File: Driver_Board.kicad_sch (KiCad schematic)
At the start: 26 parts, among them J1 200, J2 100, J3 10, J4 Conn_01x04, J5 Conn_01x04, J6 Control

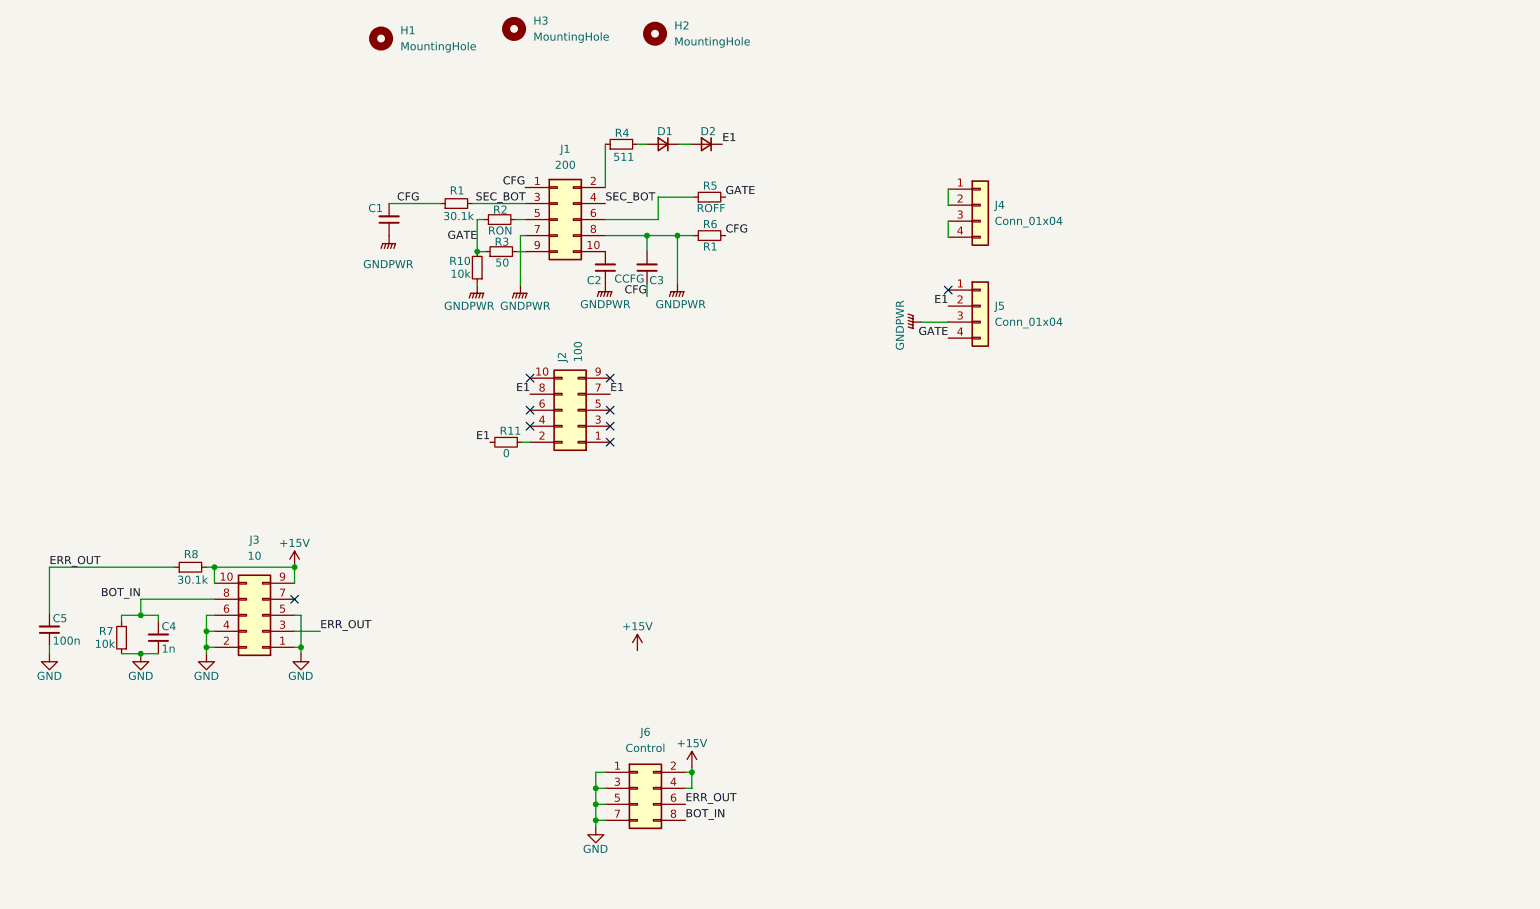
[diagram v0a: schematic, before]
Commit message: Основа ADUM4135
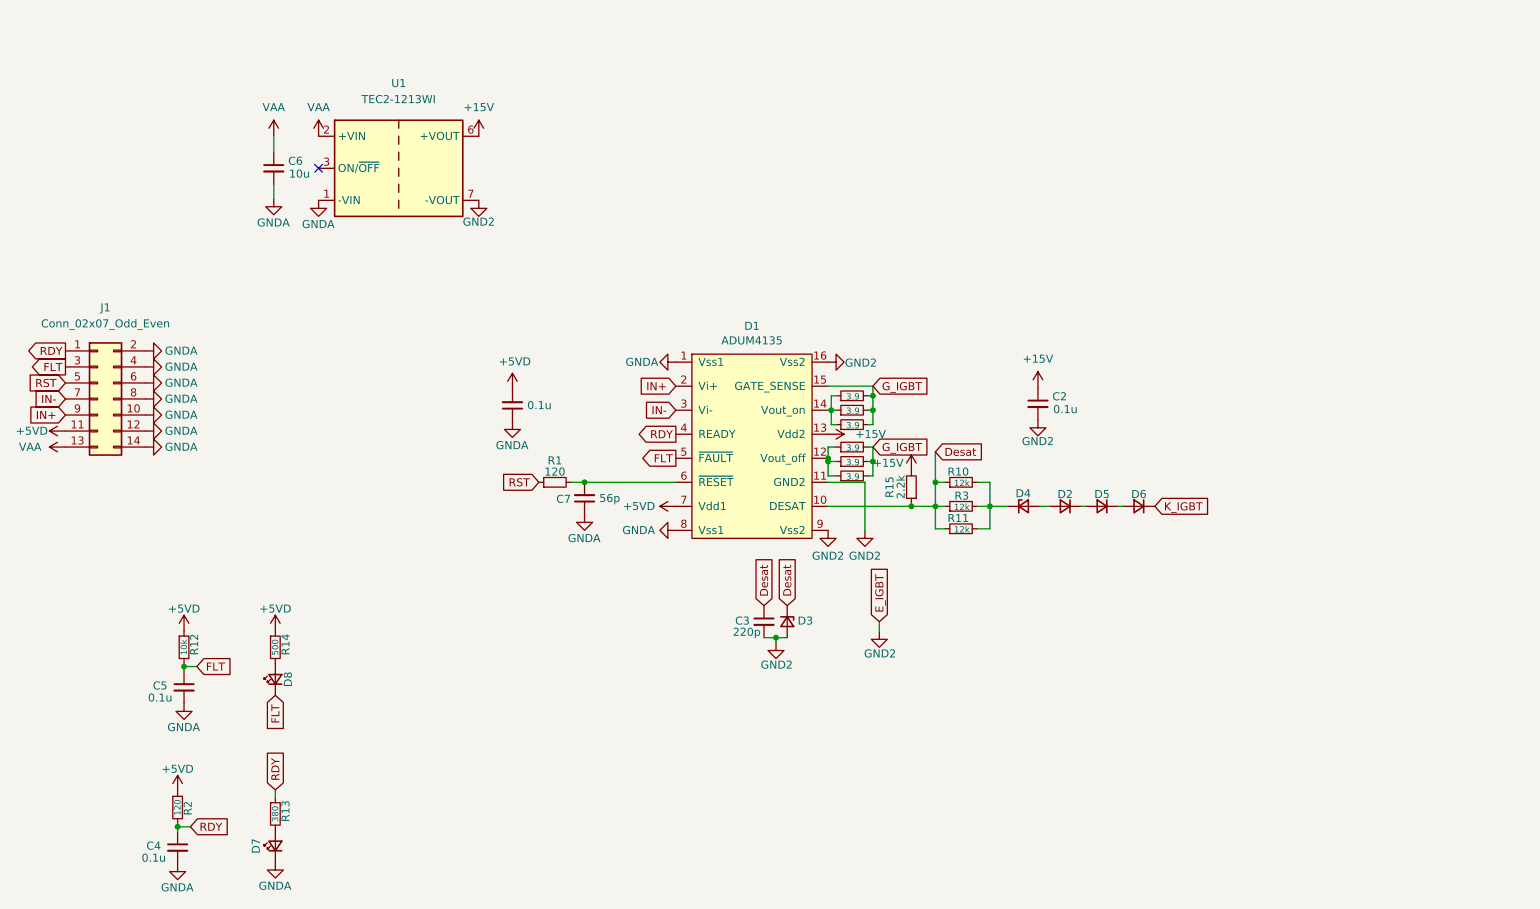
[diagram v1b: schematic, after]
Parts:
- removed D1: D_Small, Diode_SMD:D_SMA_Handsoldering, symbol Device:D_Small
- removed H1, H2, H3: MountingHole, MountingHole:MountingHole_3.2mm_M3, symbol Mechanical:MountingHole
- removed J1: 200, Connector_PinSocket_2.54mm:PinSocket_2x05_P2.54mm_Vertical, symbol Connector_Generic:Conn_02x05_Odd_Even
- removed J2: 100, Connector_PinSocket_2.54mm:PinSocket_2x05_P2.54mm_Vertical, symbol Connector_Generic:Conn_02x05_Odd_Even
- removed J3: 10, Connector_PinSocket_2.54mm:PinSocket_2x05_P2.54mm_Vertical, symbol Connector_Generic:Conn_02x05_Odd_Even
- removed J4, J5: Conn_01x04, IGBT_Modul:IGBT_Control, symbol Connector_Generic:Conn_01x04
- removed J6: Control, Connector_IDC:IDC-Header_2x04_P2.54mm_Vertical, symbol Connector_Generic:Conn_02x04_Odd_Even
- added C6: 10u, Capacitor_SMD:C_1210_3225Metric_Pad1.33x2.70mm_HandSolder, symbol Device:C_Small
- added C7: 56p, Capacitor_SMD:C_0805_2012Metric_Pad1.18x1.45mm_HandSolder, symbol Device:C_Small
- added D1: ADUM4135, Package_SO:SOIC-16W_7.5x10.3mm_P1.27mm, symbol ADUM_Driver:ADUM4135
- added D3, D4: BZT52C10-7-F, Diode_SMD:D_SOD-123, symbol Device:D_Zener_Small
- added D5, D6: MURS360T3G, Diode_SMD:D_SMA_Handsoldering, symbol Device:D_Small
- added D7, D8: LED_Small, LED_SMD:LED_0805_2012Metric_Pad1.15x1.40mm_HandSolder, symbol Device:LED_Small
- added J1: Conn_02x07_Odd_Even, Connector_IDC:IDC-Header_2x07-1MP_P2.54mm_Latch_Vertical, symbol Connector_Generic:Conn_02x07_Odd_Even
- added R12: 10k, Resistor_SMD:R_0805_2012Metric_Pad1.20x1.40mm_HandSolder, symbol Device:R_Small
- added R13: 380, Resistor_SMD:R_0805_2012Metric_Pad1.20x1.40mm_HandSolder, symbol Device:R_Small
- added R14: 500, Resistor_SMD:R_0805_2012Metric_Pad1.20x1.40mm_HandSolder, symbol Device:R_Small
- added R15: 2.2k, Resistor_SMD:R_0805_2012Metric_Pad1.20x1.40mm_HandSolder, symbol Device:R_Small
- added R9: 3.9, Resistor_SMD:R_1206_3216Metric_Pad1.30x1.75mm_HandSolder, symbol Device:R_Small
- added U1: TEC2-1213WI, Converter_DCDC:Converter_DCDC_TRACO_TMR-xxxx_THT, symbol Converter_DCDC:TEC2-1213WI
- C1, C2: value C_Small -> 0.1u
- C3: value CCFG -> 220p
- C4: value 1n -> 0.1u
- C5: value 100n -> 0.1u
- D2: value D_Small -> MURS360T3G
- R1: value 30.1k -> 120; footprint Resistor_SMD:R_2512_6332Metric_Pad1.40x3.35mm_HandSolder -> Resistor_SMD:R_0805_2012Metric_Pad1.20x1.40mm_HandSolder
- R10: value 10k -> 12k; footprint Resistor_SMD:R_2512_6332Metric_Pad1.40x3.35mm_HandSolder -> Resistor_SMD:R_1206_3216Metric_Pad1.30x1.75mm_HandSolder
- R11: value 0 -> 12k; footprint Resistor_SMD:R_2512_6332Metric_Pad1.40x3.35mm_HandSolder -> Resistor_SMD:R_1206_3216Metric_Pad1.30x1.75mm_HandSolder
- R2: value RON -> 120; footprint Resistor_SMD:R_2512_6332Metric_Pad1.40x3.35mm_HandSolder -> Resistor_SMD:R_0805_2012Metric_Pad1.20x1.40mm_HandSolder
- R3: value 50 -> 12k; footprint Resistor_SMD:R_2512_6332Metric_Pad1.40x3.35mm_HandSolder -> Resistor_SMD:R_1206_3216Metric_Pad1.30x1.75mm_HandSolder
- R4: value 511 -> 3.9; footprint Resistor_SMD:R_2512_6332Metric_Pad1.40x3.35mm_HandSolder -> Resistor_SMD:R_1206_3216Metric_Pad1.30x1.75mm_HandSolder
- R5: value ROFF -> 3.9; footprint Resistor_SMD:R_2512_6332Metric_Pad1.40x3.35mm_HandSolder -> Resistor_SMD:R_1206_3216Metric_Pad1.30x1.75mm_HandSolder
- R6: value R1 -> 3.9; footprint Resistor_SMD:R_2512_6332Metric_Pad1.40x3.35mm_HandSolder -> Resistor_SMD:R_1206_3216Metric_Pad1.30x1.75mm_HandSolder
- R7: value 10k -> 3.9; footprint Resistor_SMD:R_2512_6332Metric_Pad1.40x3.35mm_HandSolder -> Resistor_SMD:R_1206_3216Metric_Pad1.30x1.75mm_HandSolder
- R8: value 30.1k -> 3.9; footprint Resistor_SMD:R_2512_6332Metric_Pad1.40x3.35mm_HandSolder -> Resistor_SMD:R_1206_3216Metric_Pad1.30x1.75mm_HandSolder
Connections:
- net +15V: now also C2.1, D1.13 (Vdd2), R15.2, U1.6 (+VOUT); no longer R8.2
- net GND2: now reaches C2.2
- net GND2: now also C3.2, D1.11 (GND2), D1.16 (Vss2), D1.9 (Vss2), D3.2 (A), U1.7 (-VOUT)
- net at R4.1: now also R6.1, R7.1, D1.14 (Vout_on)
- net RDY: now reaches R2.2
- net RDY: now also C4.1, D1.4 (READY), J1.1 (Pin_1), R13.1
- net at R5.1: now also R8.1, D1.12 (Vout_off), R9.1
- net at R3.2: now also R10.2, R11.2, D4.1 (K)
- net G_IGBT: now reaches R4.2
- net G_IGBT: now also R5.2, R6.2, R7.2, R8.2, D1.15 (GATE_SENSE), R9.2
- net at D2.2 (A): now also D4.2 (A)
- net Desat: now reaches R11.1
- net Desat: now also C3.1, R10.1, R3.1, D1.10 (DESAT), D3.1 (K), R15.1
- net BOT_IN renamed GNDA
- net GNDA: now also C1.1, C5.2, C6.2, C7.1, D1.1 (Vss1), D1.8 (Vss1), D7.1 (K), J1.10 (Pin_10), J1.12 (Pin_12), J1.14 (Pin_14), J1.2 (Pin_2), J1.4 (Pin_4), J1.6 (Pin_6), J1.8 (Pin_8), U1.1 (-VIN); no longer R7.2
- removed net CFG: C1.2, C3.1, R1.1, R6.2
- net E1: no longer names the net of D2.1 (K)
- net E1: now also D5.2 (A); no longer R11.2
- removed net ERR_OUT: C5.2, R8.1
- removed net GATE: R10.2, R2.1, R3.1, R5.2
- removed net GND: C4.1, C5.1, R7.1
- removed net GNDPWR: C1.1, C2.1, C3.2, R10.1, R6.1
- net SEC_BOT: no longer names the net of R1.2
- net SEC_BOT: now also C7.2, D1.6 (~{RESET})
- new net: D5.1 (K), D6.2 (A)
- new net: D7.2 (A), R13.2
- new net: D8.2 (A), R14.2
- new net +5VD: C1.2, D1.7 (Vdd1), J1.11 (Pin_11), R12.1, R14.1, R2.1
- new net FLT: C5.1, D1.5 (~{FAULT}), D8.1 (K), J1.3 (Pin_3), R12.2
- new net IN+: D1.2 (Vi+), J1.9 (Pin_9)
- new net IN-: D1.3 (Vi-), J1.7 (Pin_7)
- new net K_IGBT: D6.1 (K)
- new net RST: J1.5 (Pin_5), R1.1
- new net VAA: C6.1, J1.13 (Pin_13), U1.2 (+VIN)
- no-connect marks 9 -> 1

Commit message: Плата на два модуля
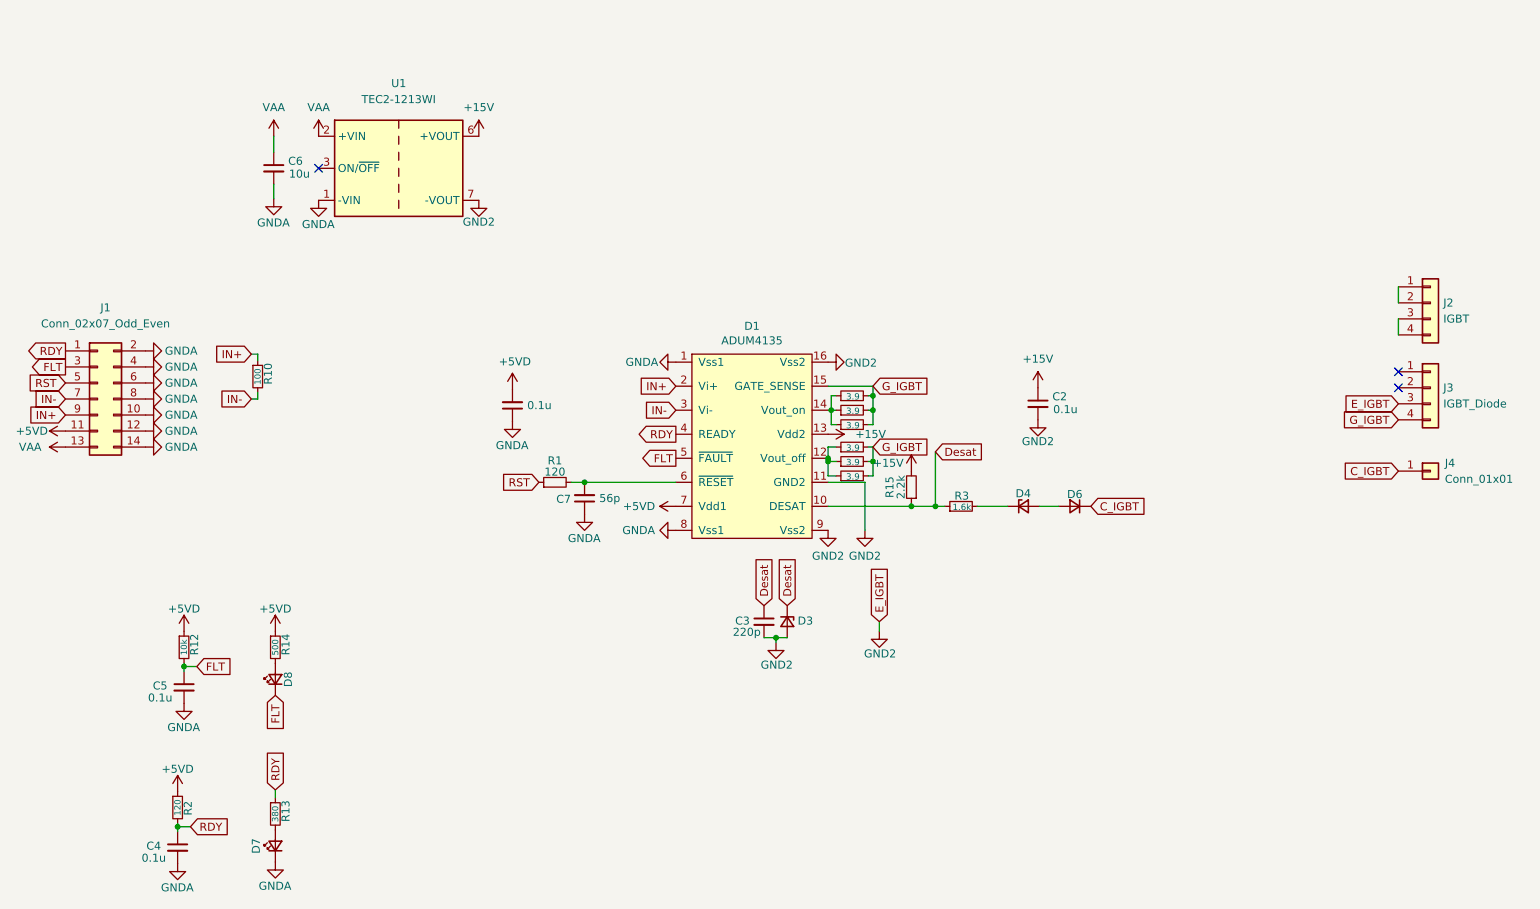
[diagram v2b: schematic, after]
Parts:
- removed D2, D5: MURS360T3G, Diode_SMD:D_SMA_Handsoldering, symbol Device:D_Small
- removed R11: 12k, Resistor_SMD:R_1206_3216Metric_Pad1.30x1.75mm_HandSolder, symbol Device:R_Small
- added J2: IGBT, IGBT_Modul:IGBT_Gate, symbol Connector_Generic:Conn_01x04
- added J3: IGBT_Diode, IGBT_Modul:IGBT_Gate, symbol Connector_Generic:Conn_01x04
- added J4: Conn_01x01, Connector Power:Wire, symbol Connector_Generic:Conn_01x01
- R10: value 12k -> 100; footprint Resistor_SMD:R_1206_3216Metric_Pad1.30x1.75mm_HandSolder -> Resistor_SMD:R_0805_2012Metric_Pad1.20x1.40mm_HandSolder
- R3: value 12k -> 1.6k
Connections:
- net Desat: no longer R10.1
- net GND2: now also J3.3 (Pin_3)
- net G_IGBT: now also J3.4 (Pin_4)
- net IN+: now also R10.1
- net IN-: now also R10.2
- net at D6.2 (A): now also D4.2 (A)
- net at D4.1 (K), R3.2: no longer R10.2
- net K_IGBT renamed C_IGBT
- net C_IGBT: now also J4.1 (Pin_1)
- new net: J2.1 (Pin_1), J2.2 (Pin_2)
- new net: J2.3 (Pin_3), J2.4 (Pin_4)
- no-connect marks 1 -> 3
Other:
- moved on the sheet: D6
